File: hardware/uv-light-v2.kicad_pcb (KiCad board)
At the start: 2 copper layers, 15 x 25 mm, 24 parts, among them P1 CON-SENSOR2, P2 DEBUG, P3 BOOT, U1 XMC1100, U2 VEML6075, U3 DRILL, U4 DRILL, U5 DRILL, U6 DRILL

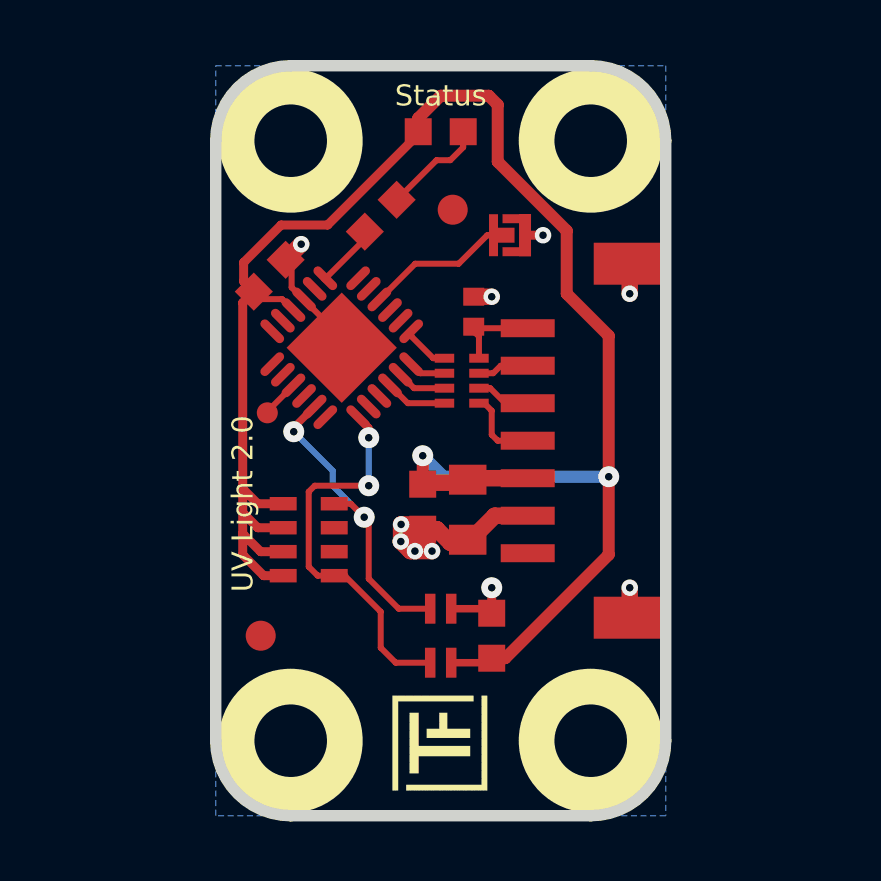
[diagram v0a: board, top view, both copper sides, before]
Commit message: Data Cleanup
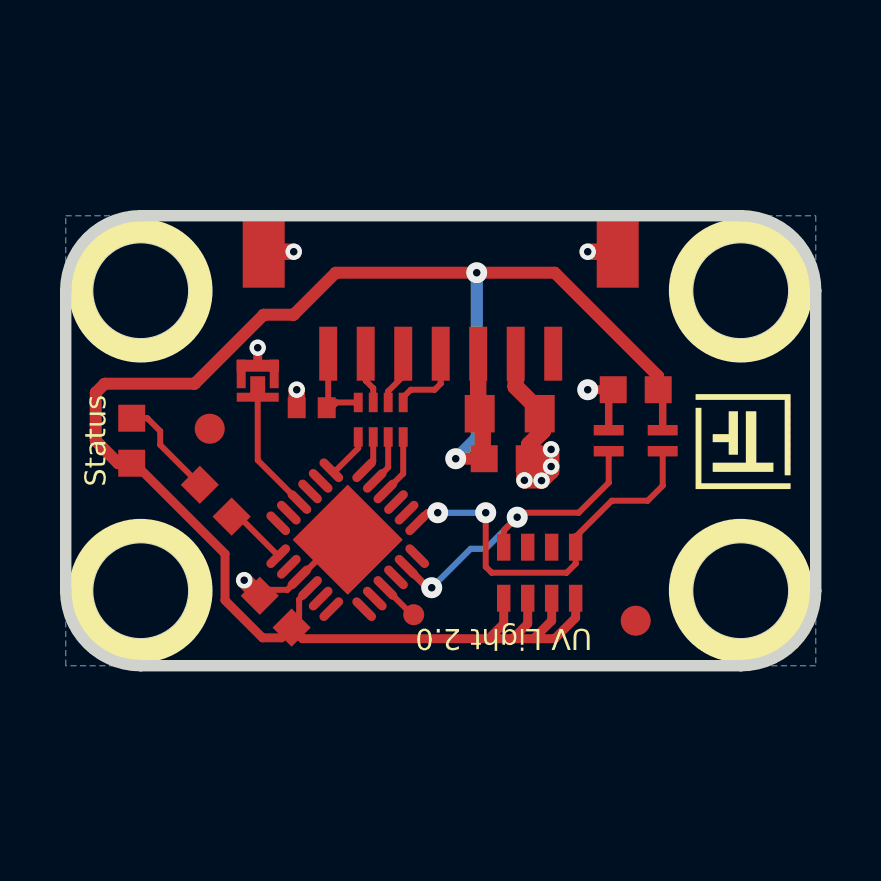
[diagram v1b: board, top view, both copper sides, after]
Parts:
- moved G*** 16.6 mm to (148.6, 89.5), turned to 180 degrees
- moved U3 15.8 mm to (126.9, 82.9), turned to 180 degrees
- moved U4 15.8 mm to (146.9, 92.9), turned to 180 degrees
- moved U5 15.8 mm to (146.9, 82.9), turned to 180 degrees
- moved U6 15.8 mm to (126.9, 92.9), turned to 180 degrees
- moved D1 14.6 mm to (126.6, 87.9), turned to 90 degrees
- moved Fiducial_Mark 12.5 mm to (143.4, 93.9), turned to 90 degrees
- moved C4 11.2 mm to (131.4, 93.6), turned to -45 degrees
- moved R1 11.0 mm to (129.4, 89.9), turned to 135 degrees
- moved Fiducial_Mark 10.9 mm to (129.2, 87.5), turned to 90 degrees
- moved P1 10.6 mm to (136.9, 80.4), turned to 180 degrees
- moved P3 9.71 mm to (130.8, 85.9), turned to -90 degrees
- moved C5 9.50 mm to (143.4, 86.2), turned to 0 degrees
- moved U2 9.19 mm to (143.4, 87.9), turned to 0 degrees
- moved VAL 8.49 mm to (142.9, 87.9), turned to 0 degrees
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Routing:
- net GND: track 25.3 -> 23.8 mm
- net Net-(P3-Pad2): track 5.20 -> 4.17 mm
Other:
- board size 15 x 25 mm -> 25 x 15 mm
- net class Default removed
- board text added: "Copyright Tinkerforge GmbH 2023. This documentation describes Open Hardware and is licensed under the CERN OHL v. 1.1. You may redistribute and modify this documentation under the terms of the CERN OHL v.1.1. (http://ohwr.org/cernohl). This documentation is distributed WITHOUT ANY EXPRESS OR IMPLIED WARRANTY, INCLUDING OF MERCHANTABILITY, SATISFACTORY QUALITY AND FITNESS FOR A PARTICULAR PURPOSE.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"
- board text removed: "Copyright Tinkerforge GmbH 2018. This documentation describes Open Hardware and is licensed under the CERN OHL v. 1.1. You may redistribute and modify this documentation under the terms of the CERN OHL v.1.1. (http://ohwr.org/cernohl). This documentation is distributed WITHOUT ANY EXPRESS OR IMPLIED WARRANTY, INCLUDING OF MERCHANTABILITY, SATISFACTORY QUALITY AND FITNESS FOR A PARTICULAR PURPOSE.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"
